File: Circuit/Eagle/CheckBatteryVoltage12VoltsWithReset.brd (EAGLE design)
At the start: 100.3 x 70 mm, 147 parts

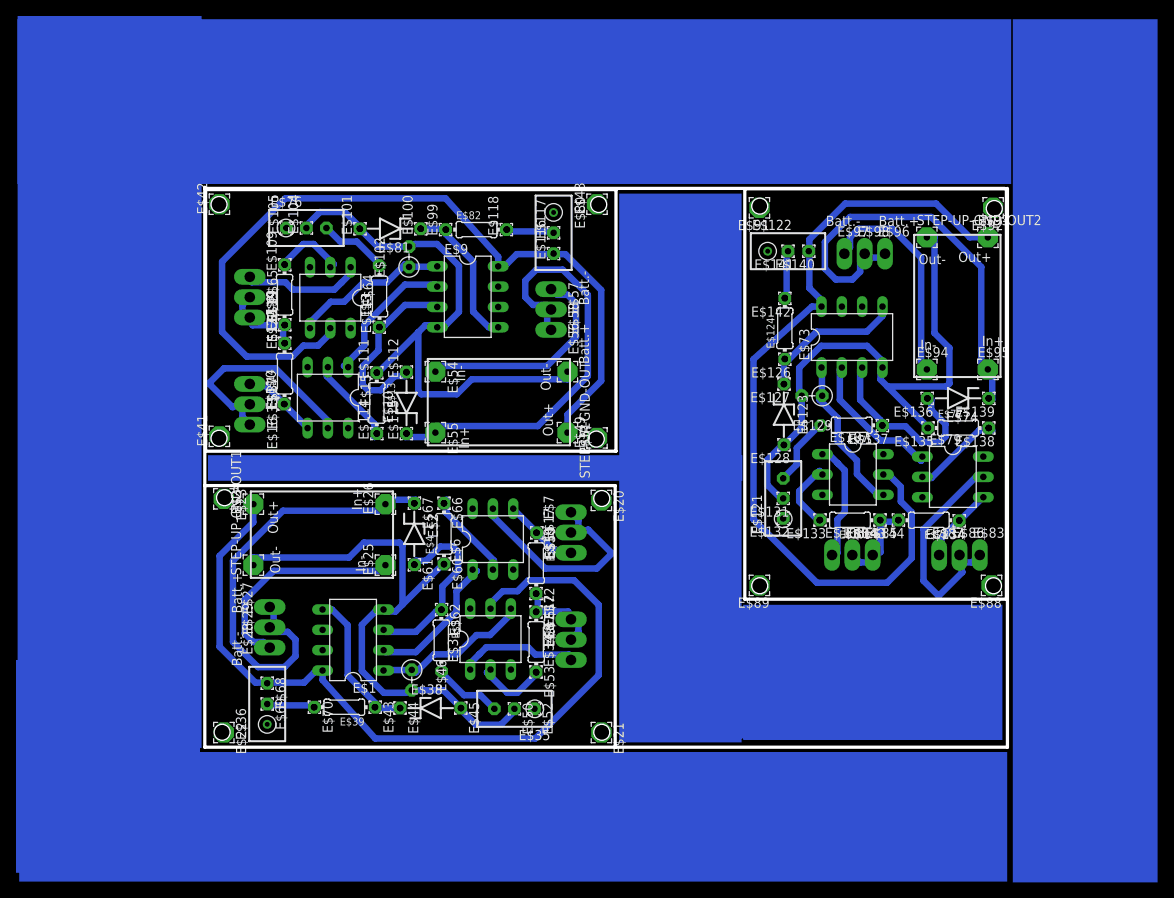
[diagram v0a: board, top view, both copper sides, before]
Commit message: .
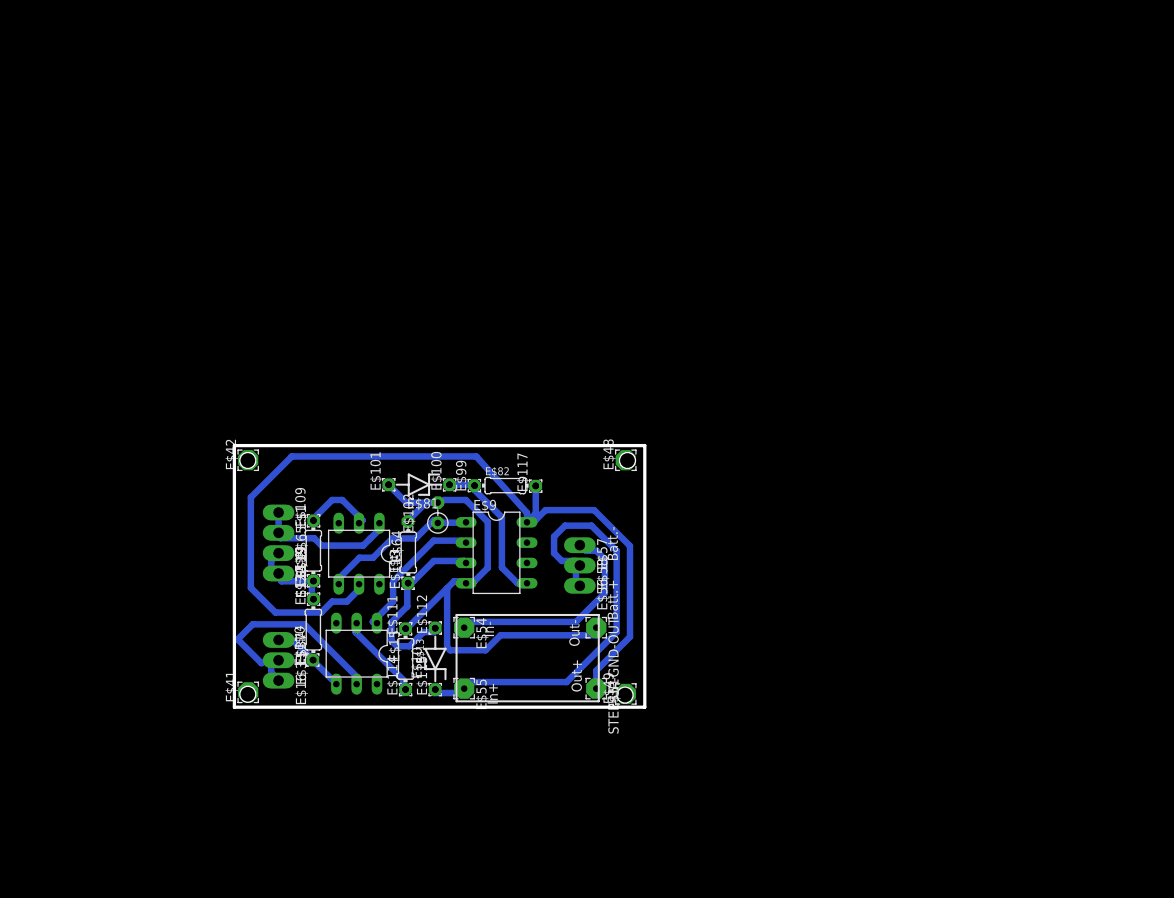
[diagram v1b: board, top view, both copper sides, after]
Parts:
- removed E$103, E$104, E$105, E$116, E$118, E$125, E$126, E$127, E$128, E$130, E$131, E$132, E$133, E$134, E$135, E$136, E$137, E$138, E$139, E$140, E$141, E$142, E$143, E$144, E$40, E$43, E$44, E$45, E$47, E$50, E$52, E$53, E$59, E$60, E$61, E$62, E$66, E$67, E$68, E$69, E$70, E$71, E$72: (no value), wirepad:1,6/0,8
- removed E$106, E$30, E$4, E$5, E$77, E$78: 220, eagle-ltspice:0204/7
- removed E$107, E$31, E$6, E$79: Til113, ic-package:DIL06
- removed E$108, E$12, E$17, E$18, E$27, E$28, E$29, E$34, E$7, E$8, E$83, E$84, E$85, E$86, E$87, E$96, E$97, E$98: (no value), testpad:P1-13Y
- removed E$121, E$35, E$76: W203, rcl:RTRIM3296W
- removed E$122, E$36, E$80: w501, rcl:RTRIM3296W
- removed E$123, E$38: zener 4.3v, ref-packages-longpad:ZDIO-7.5
- removed E$124, E$39: 100, eagle-ltspice:0204/7
- removed E$129, E$46: (no value), discrete:RS-2,5
- removed E$2, E$74: zener 10v, ref-packages-longpad:ZDIO-7.5
- removed E$20, E$21, E$22, E$23, E$24, E$25, E$26, E$88, E$89, E$91, E$92, E$93, E$94, E$95, STEP-UP-GND-OUT1, STEP-UP-GND-OUT2: (no value), wirepad:2,54/0,8
- removed E$3, E$75: 680, eagle-ltspice:0204/7
- removed E$73: Attiny85, 74xx-us:DIL08
- E$1: value Attiny85 -> (none); device 74xx-us:DIL08 -> testpad:P1-13Y
- E$102: value (none) -> 220
- E$11: value 680 -> 220
- E$81: value zener 4.3v -> zener 3.6v
- E$82: value 100 -> 47
- moved E$42 32.2 mm to (5.42, 35.9)
- moved E$48 32.2 mm to (52.6, 35.9)
- moved E$100 32.2 mm to (30.6, 32.8)
- moved E$101 32.2 mm to (23.0, 32.8)
- moved E$11 32.2 mm to (25.4, 24.3)
- moved E$110 32.2 mm to (13.5, 10.9)
- moved E$112 32.2 mm to (28.8, 14.9)
- moved E$113 32.2 mm to (25.4, 20.5)
- moved E$114 32.2 mm to (25.1, 7.20)
- moved E$115 32.2 mm to (28.8, 7.20)
- moved E$120 32.2 mm to (13.6, 18.5)
- moved E$14 32.2 mm to (13.6, 14.7)
- moved E$15 32.2 mm to (19.0, 11.7)
- moved E$16 32.2 mm to (9.22, 8.32)
- moved E$19 32.2 mm to (9.22, 24.3)
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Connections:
- removed net 5.1V-STEP-UP1: E$1.8, E$24.1, E$31.5, E$36.3
- removed net 5.1V-STEP-UP2: E$107.5, E$122.3, E$73.8, E$93.1
- removed net IN-12V-BATTERY1: E$2.C, E$26.1, E$27.TP, E$29.TP
- removed net IN-12V-BATTERY2: E$74.C, E$95.1, E$96.TP, E$98.TP
- removed net IN-5V-FROM-NANO-SDCARD1: E$17.TP, E$6.5, E$7.TP
- removed net IN-5V-FROM-NANO-SDCARD2: E$79.5, E$83.TP, E$86.TP
- removed net IN-GND-BATTERY1: E$25.1, E$28.TP
- removed net IN-GND-BATTERY2: E$94.1, E$97.TP
- removed net IN-GND-NANO-SD-CARD1: E$12.TP, E$30.1, E$5.2, E$8.TP
- removed net IN-GND-NANO-SD-CARD2: E$106.1, E$78.2, E$84.TP, E$85.TP
- removed net IN-TO-RESET-ATTINY1: E$31.1, E$34.TP
- removed net IN-TO-RESET-ATTINY2: E$107.1, E$108.TP
- removed net OUT-SERIAL-DATA1: E$18.TP, E$5.1, E$6.4
- removed net OUT-SERIAL-DATA2: E$78.1, E$79.4, E$87.TP
- removed net PHOTO-DIODE1: E$4.2, E$6.2
- removed net PHOTO-DIODE2: E$77.2, E$79.2
- removed net S$10: E$122.2, E$124.2
- removed net S$11: E$107.4, E$129.1, E$73.1
- removed net S$17: E$11.2, E$76.3
- removed net S$18: E$80.2, E$82.2
- removed net S$2: E$30.2, E$31.2
- removed net S$3: E$3.2, E$35.3
- removed net S$4: E$36.2, E$39.2
- removed net S$7: E$1.1, E$31.4, E$46.1
- removed net S$8: E$106.2, E$107.2
- removed net S$9: E$121.3, E$75.2
- removed net STEP-UP-GND1: E$1.4, E$35.2, E$38.A, E$4.1, E$46.2, STEP-UP-GND-OUT1.1
- removed net STEP-UP-GND2: E$121.2, E$123.A, E$129.2, E$73.4, E$77.1, STEP-UP-GND-OUT2.1
- removed net TX-SERIAL-DATA1: E$1.2, E$6.1
- removed net TX-SERIAL-DATA2: E$73.2, E$79.1
- removed net VZ-ANALOG-REFERENCE1: E$1.5, E$38.C, E$39.1
- removed net VZ-ANALOG-REFERENCE2: E$123.C, E$124.1, E$73.5
- removed net VZ-BATTERY-LEVEL1: E$1.3, E$2.A, E$3.1
- removed net VZ-BATTERY-LEVEL2: E$73.3, E$74.A, E$75.1
- net 5.1V-STEP-UP: now also E$82.2; no longer E$80.3
- net IN-TO-RESET-ATTINY85: now also E$1.TP
- net STEP-UP-GND: now also E$11.2; no longer E$76.2
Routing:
- net 5.1V-STEP-UP2: track 103.2 -> 0.00 mm
- net 5.1V-STEP-UP1: track 103.2 -> 0.00 mm
- net STEP-UP-GND2: track 70.5 -> 0.00 mm
- net STEP-UP-GND1: track 70.5 -> 0.00 mm
- net IN-12V-BATTERY2: track 56.0 -> 0.00 mm
- net IN-12V-BATTERY1: track 56.0 -> 0.00 mm
- net IN-5V-FROM-NANO-SDCARD1: track 28.7 -> 0.00 mm
- net IN-5V-FROM-NANO-SDCARD2: track 28.7 -> 0.00 mm
- net IN-GND-BATTERY2: track 27.8 -> 0.00 mm
- net IN-GND-BATTERY1: track 27.8 -> 0.00 mm
- net VZ-BATTERY-LEVEL1: track 23.4 -> 0.00 mm
- net VZ-BATTERY-LEVEL2: track 23.4 -> 0.00 mm
- net S$7: track 19.7 -> 0.00 mm
- net S$11: track 19.7 -> 0.00 mm
- net VZ-ANALOG-REFERENCE1: track 18.9 -> 0.00 mm
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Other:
- board size 100.3 x 70 mm -> 51.3 x 32.7 mm
